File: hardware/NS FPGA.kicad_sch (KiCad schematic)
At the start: 42 parts, among them J1 USB_C_Receptacle_USB2.0_14P, J2 Conn_01x24_Pin, J3 Conn_01x24_Pin, J4 Jtag PIN, Q1 BSS138, SW1 SW_Push, U2 CP2102N-Axx-xQFN24, U3 AP2112K-3.3, U4 AP2112K-1.2, Y1 SG-8002CE(24.0000M)

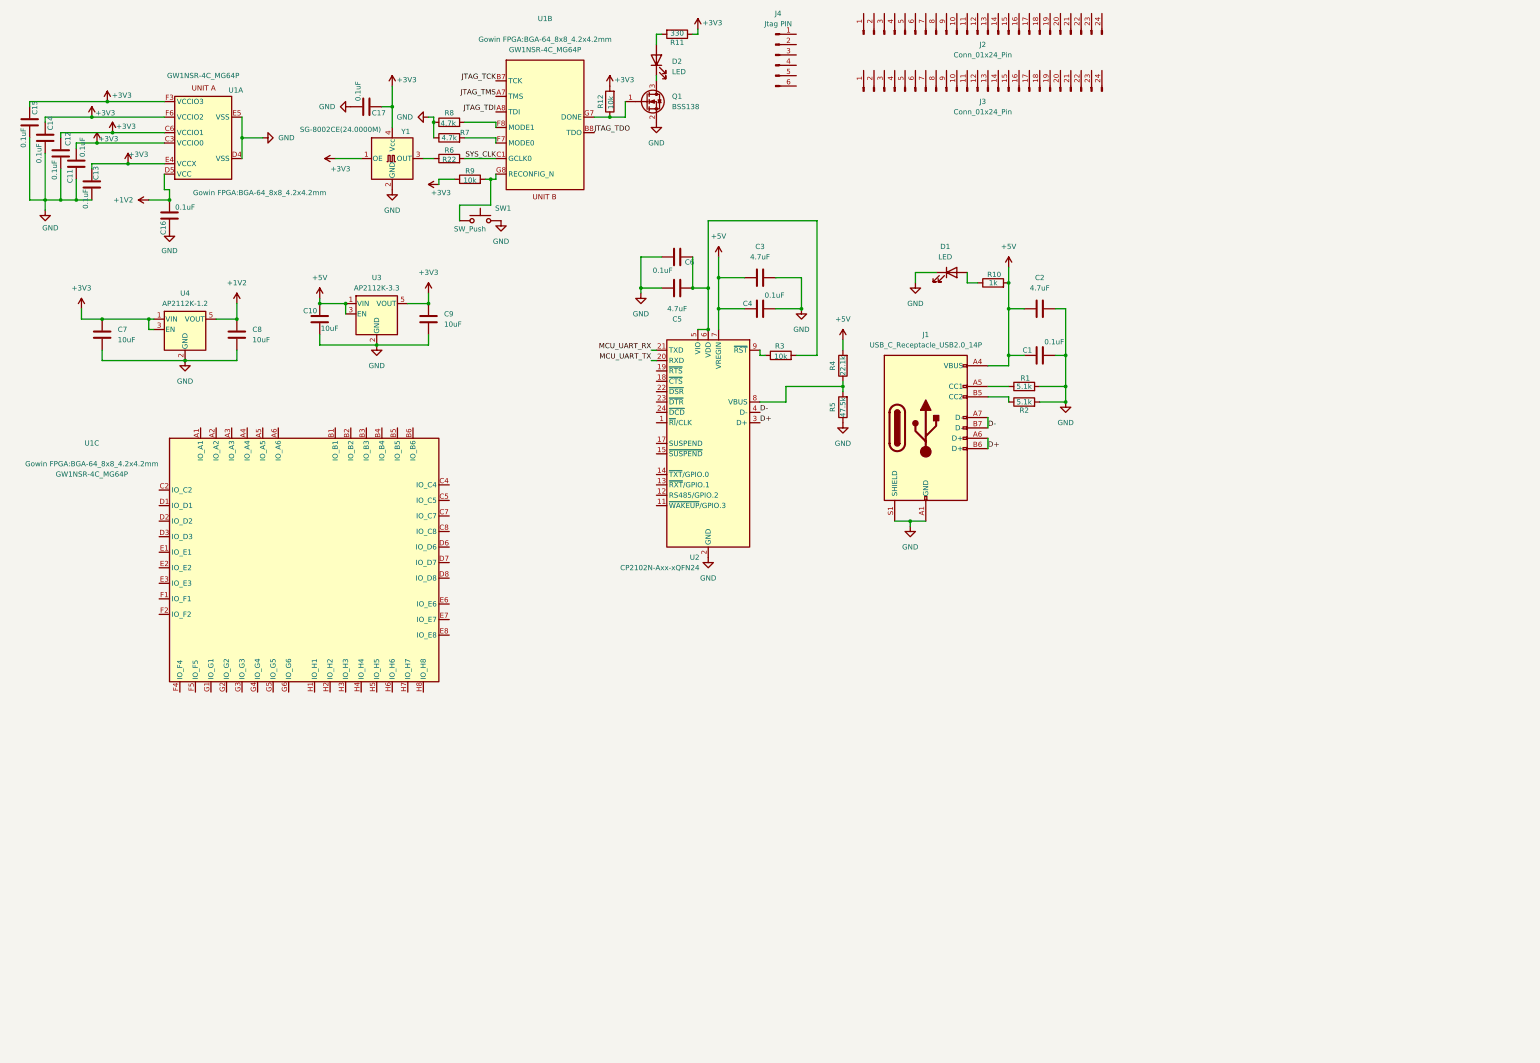
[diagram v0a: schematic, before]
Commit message: push
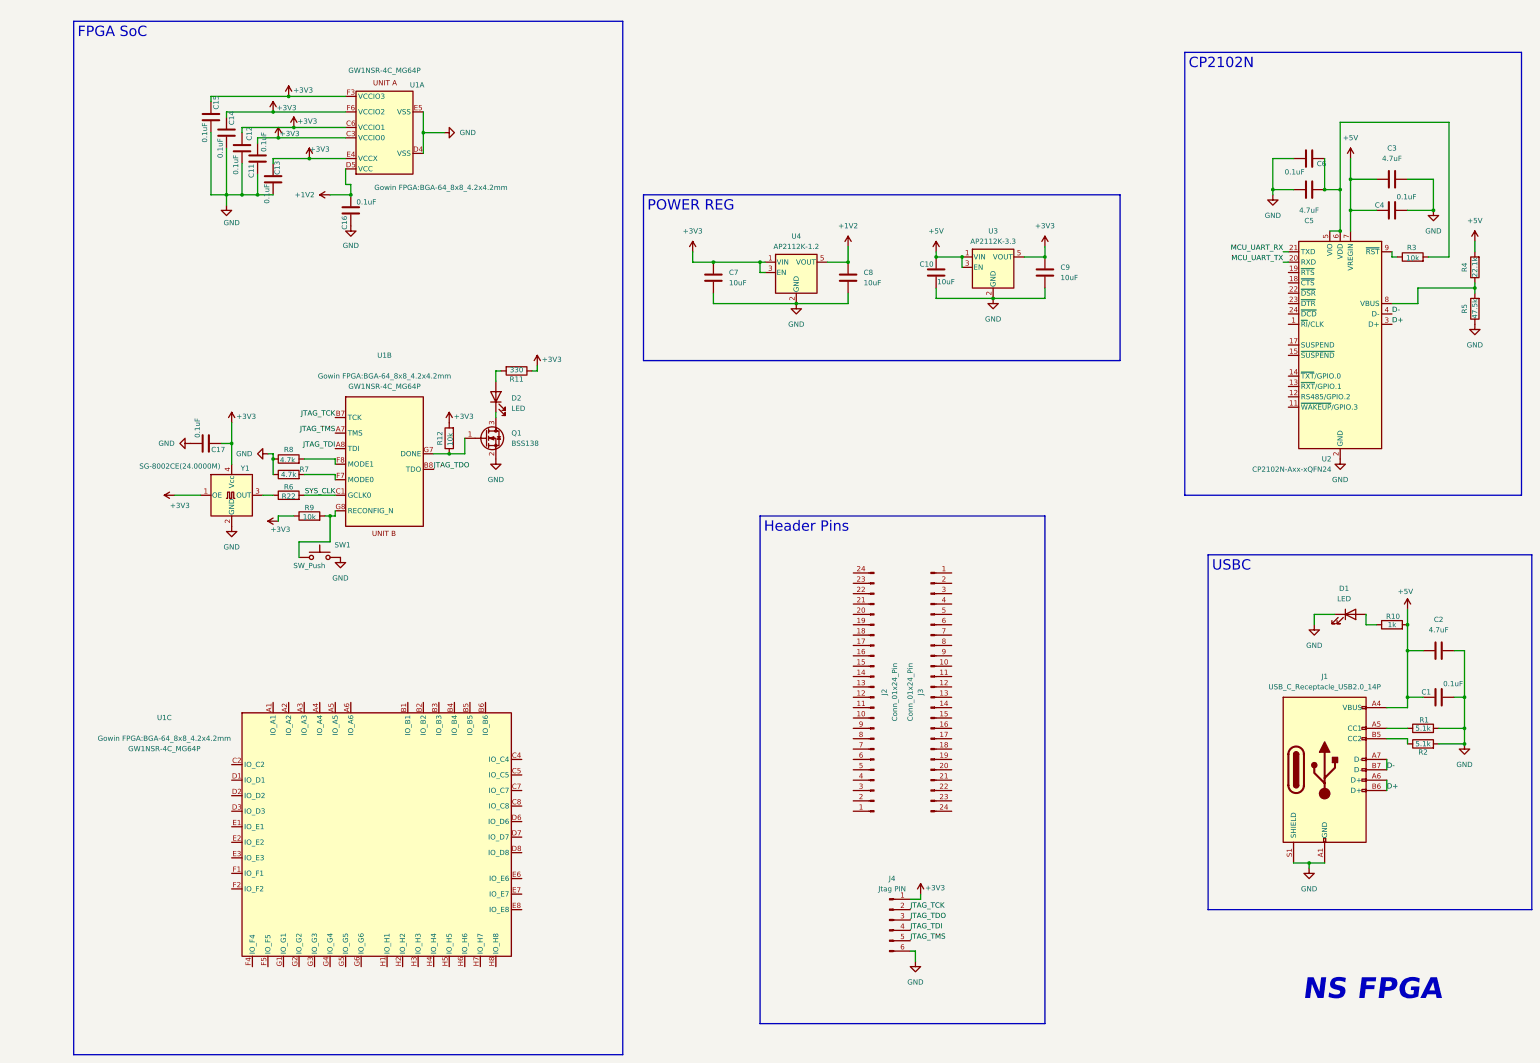
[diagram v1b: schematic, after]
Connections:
- net +3V3: now also J4.1 (Pin_1)
- net GND: now also J4.6 (Pin_6)
- net JTAG_TCK: now also J4.2 (Pin_2)
- net JTAG_TDI: now also J4.4 (Pin_4)
- net JTAG_TDO: now also J4.3 (Pin_3)
- net JTAG_TMS: now also J4.5 (Pin_5)
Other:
- note added: "NS FPGA"
- moved on the sheet: C1, C10, C11, C12, C13, C14, C15, C16, C17, C2, C3, C4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
